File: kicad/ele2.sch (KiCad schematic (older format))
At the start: 3 parts, among them SW1 SW_Push, U1 WeMos_D1_mini, U2 HX711_module

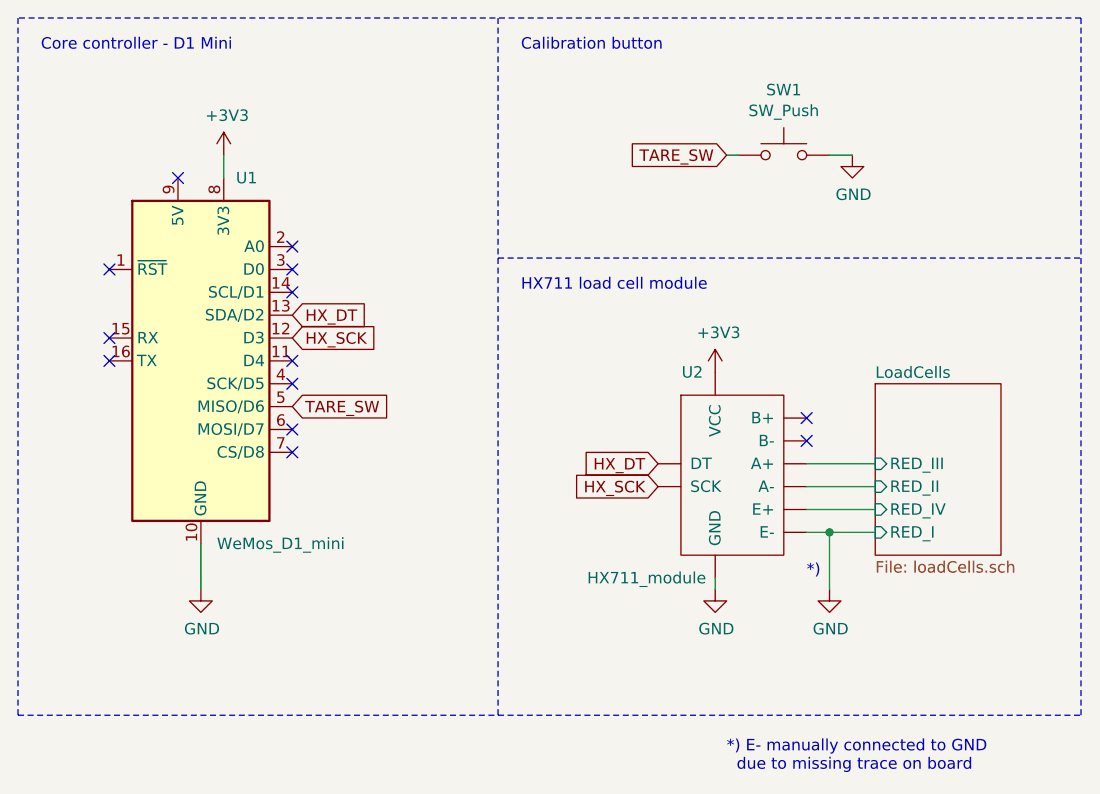
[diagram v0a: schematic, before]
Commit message: Update schematic
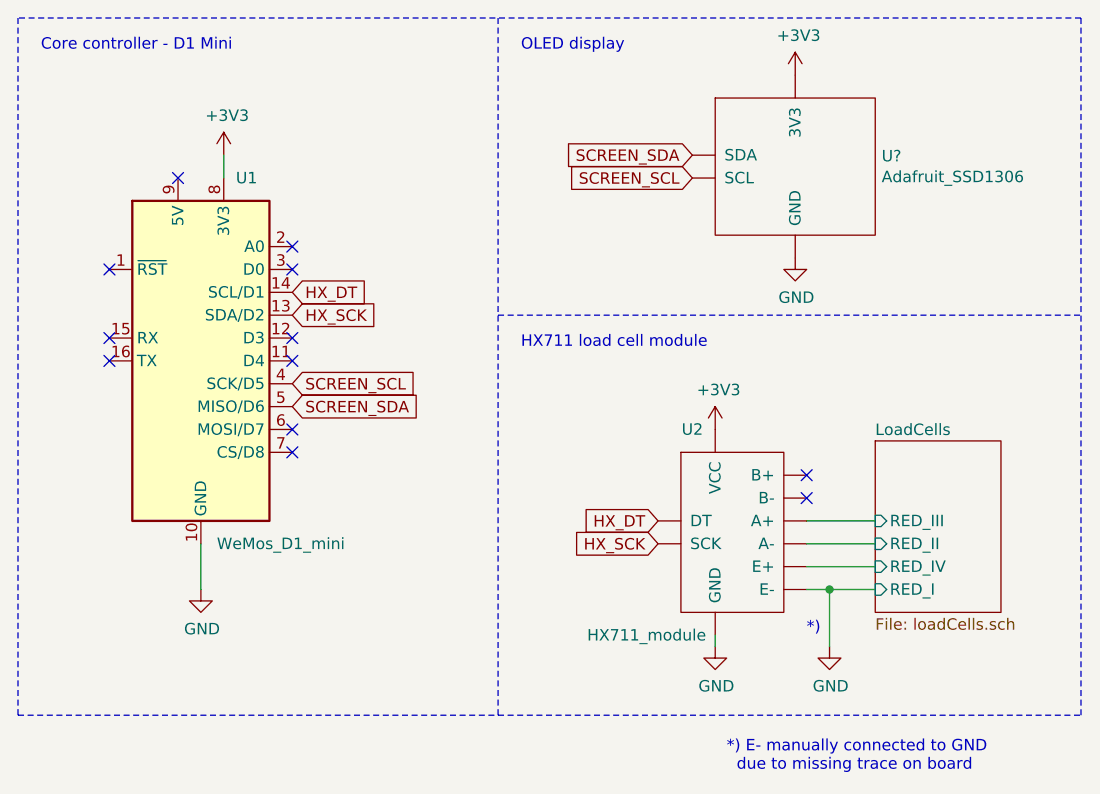
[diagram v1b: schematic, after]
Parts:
- removed SW1: SW_Push, symbol Switch:SW_Push
- added U?: Adafruit_SSD1306, symbol ele2:Adafruit_SSD1306
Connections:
- net +3V3: now also U?.~ (SDA)
- net GND: now also U?.~ (SDA)
- net HX_DT: now also U1.14 (SCL/D1); no longer U1.13 (SDA/D2)
- net HX_SCK: now also U1.13 (SDA/D2); no longer U1.12 (D3)
- net SCREEN_SCL: now reaches U1.4 (SCK/D5)
- net SCREEN_SCL: now also U?.~ (SDA)
- net TARE_SW renamed SCREEN_SDA
- net SCREEN_SDA: now also U?.~ (SDA)
- no-connect marks 13 -> 12
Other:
- note added: "OLED display"
- note removed: "Calibration button"
- moved on the sheet: U2
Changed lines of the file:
@@
 	4250 4950 4250 4750
-$Comp
-L Switch:SW_Push SW1
-U 1 1 5E80F0CB
-P 6800 3050
-F 0 "SW1" H 6800 3335 50  0000 C CNN
-F 1 "SW_Push" H 6800 3244 50  0000 C CNN
-F 2 "" H 6800 3250 50  0001 C CNN
-F 3 "~" H 6800 3250 50  0001 C CNN
-	1    6800 3050
-	1    0    0    -1
-$EndComp
-$Comp
-L power:GND #PWR?
-U 1 1 5E81082F
-P 7100 3050
-F 0 "#PWR?" H 7100 2800 50  0001 C CNN
-F 1 "GND" H 7105 2877 50  0000 C CNN
-F 2 "" H 7100 3050 50  0001 C CNN
-F 3 "" H 7100 3050 50  0001 C CNN
-	1    7100 3050
-	1    0    0    -1
-$EndComp
-Wire Wire Line
-	6550 3050 6600 3050
-Wire Wire Line
-	7000 3050 7100 3050
 $Comp
 L ele2:HX711_module U2
 U 1 1 5E815E00
-P 6550 4450
-F 0 "U2" H 6400 4900 50  0000 C CNN
-F 1 "HX711_module" H 6200 4000 50  0000 C CNN
-F 2 "" H 6550 4450 50  0001 C CNN
-F 3 "" H 6550 4450 50  0001 C CNN
-	1    6550 4450
-	1    0    0    -1
-$EndComp
-$Comp
-L power:+3V3 #PWR?
-U 1 1 5E81AC21
-P 6500 4000
-F 0 "#PWR?" H 6500 3850 50  0001 C CNN
-F 1 "+3V3" H 6515 4173 50  0000 C CNN
-F 2 "" H 6500 4000 50  0001 C CNN
-F 3 "" H 6500 4000 50  0001 C CNN
-	1    6500 4000
+P 6550 4700
+F 0 "U2" H 6400 5150 50  0000 C CNN
+F 1 "HX711_module" H 6200 4250 50  0000 C CNN
+F 2 "" H 6550 4700 50  0001 C CNN
+F 3 "" H 6550 4700 50  0001 C CNN
+	1    6550 4700
 	1    0    0    -1
 $EndComp
@@
 L power:GND #PWR?
 U 1 1 5E81C444
-P 6500 4950
-F 0 "#PWR?" H 6500 4700 50  0001 C CNN
-F 1 "GND" H 6505 4777 50  0000 C CNN
-F 2 "" H 6500 4950 50  0001 C CNN
-F 3 "" H 6500 4950 50  0001 C CNN
-	1    6500 4950
+P 6500 5200
+F 0 "#PWR?" H 6500 4950 50  0001 C CNN
+F 1 "GND" H 6505 5027 50  0000 C CNN
+F 2 "" H 6500 5200 50  0001 C CNN
+F 3 "" H 6500 5200 50  0001 C CNN
+	1    6500 5200
 	1    0    0    -1
 $EndComp
 Wire Wire Line
-	6500 4900 6500 4950
+	6500 5150 6500 5200
 NoConn ~ 4650 3450
 NoConn ~ 4650 3550
-NoConn ~ 4650 3650
-NoConn ~ 4650 4050
 NoConn ~ 4650 3950
-Text GLabel 6550 3050 0    50   Input ~ 0
-TARE_SW
-Text GLabel 4650 4150 2    50   Input ~ 0
-TARE_SW
+Text GLabel 4650 4050 2    50   Input ~ 0
+SCREEN_SCL
 NoConn ~ 4650 4250
 NoConn ~ 4650 4350
+Text GLabel 4650 3650 2    50   Input ~ 0
+HX_DT
+Text GLabel 6250 4750 0    50   Input ~ 0
+HX_SCK
 Text GLabel 4650 3750 2    50   Input ~ 0
-HX_DT
-Text GLabel 6250 4500 0    50   Input ~ 0
 HX_SCK
-Text GLabel 4650 3850 2    50   Input ~ 0
-HX_SCK
-Text GLabel 6250 4400 0    50   Input ~ 0
+Text GLabel 6250 4650 0    50   Input ~ 0
 HX_DT
 Wire Notes Line
@@
 	5550 2450 5550 5500
 Wire Notes Line
-	5550 3500 8100 3500
-Text Notes 5650 2600 0    50   ~ 0
-Calibration button
-Text Notes 5650 3650 0    50   ~ 0
+	5550 3750 8100 3750
+Text Notes 5650 3900 0    50   ~ 0
 HX711 load cell module
 Text Notes 3550 2600 0    50   ~ 0
 Core controller - D1 Mini
 Wire Wire Line
-	6900 4700 7000 4700
-Connection ~ 7000 4700
+	6900 4950 7000 4950
+Connection ~ 7000 4950
 $Comp
 L power:GND #PWR?
 U 1 1 5E83F78A
-P 7000 4950
-F 0 "#PWR?" H 7000 4700 50  0001 C CNN
-F 1 "GND" H 7005 4777 50  0000 C CNN
-F 2 "" H 7000 4950 50  0001 C CNN
-F 3 "" H 7000 4950 50  0001 C CNN
-	1    7000 4950
+P 7000 5200
+F 0 "#PWR?" H 7000 4950 50  0001 C CNN
+F 1 "GND" H 7005 5027 50  0000 C CNN
+F 2 "" H 7000 5200 50  0001 C CNN
+F 3 "" H 7000 5200 50  0001 C CNN
+	1    7000 5200
 	1    0    0    -1
 $EndComp
 Wire Wire Line
-	7000 4700 7000 4950
-Text Notes 6900 4900 0    50   ~ 0
+	7000 4950 7000 5200
+Text Notes 6900 5150 0    50   ~ 0
 *)
 Text Notes 6550 5750 0    50   ~ 0
 *) E- manually connected to GND\n  due to missing trace on board
 $Sheet
-S 7200 4050 550  750
+S 7200 4300 550  750
 U 5E83A8FB
 F0 "LoadCells" 50
 F1 "loadCells.sch" 50
-F2 "RED_II" I L 7200 4500 50
-F3 "RED_I" I L 7200 4700 50
-F4 "RED_IV" I L 7200 4600 50
-F5 "RED_III" I L 7200 4400 50
+F2 "RED_II" I L 7200 4750 50
+F3 "RED_I" I L 7200 4950 50
+F4 "RED_IV" I L 7200 4850 50
+F5 "RED_III" I L 7200 4650 50
 $EndSheet
-NoConn ~ 6900 4200
-NoConn ~ 6900 4300
+NoConn ~ 6900 4450
+NoConn ~ 6900 4550
 Wire Wire Line
-	6900 4400 7200 4400
+	6900 4650 7200 4650
 Wire Wire Line
-	6900 4500 7200 4500
+	6900 4750 7200 4750
 Wire Wire Line
-	6900 4600 7200 4600
+	6900 4850 7200 4850
 Wire Wire Line
-	7000 4700 7200 4700
+	7000 4950 7200 4950
+NoConn ~ 4650 3850
+Text GLabel 4650 4150 2    50   Input ~ 0
+SCREEN_SDA
+$Comp
+L ele2:Adafruit_SSD1306 U?
+U 1 1 5EBEA0D0
+P 6750 3100
+F 0 "U?" H 7228 3146 50  0000 L CNN
+F 1 "Adafruit_SSD1306" H 7228 3055 50  0000 L CNN
+F 2 "" H 6750 3050 50  0001 C CNN
+F 3 "" H 6750 3050 50  0001 C CNN
+	1    6750 3100
+	1    0    0    -1
+$EndComp
+$Comp
+L power:+3V3 #PWR?
+U 1 1 5E81AC21
+P 6500 4250
+F 0 "#PWR?" H 6500 4100 50  0001 C CNN
+F 1 "+3V3" H 6515 4423 50  0000 C CNN
+F 2 "" H 6500 4250 50  0001 C CNN
+F 3 "" H 6500 4250 50  0001 C CNN
+	1    6500 4250
+	1    0    0    -1
+$EndComp
+$Comp
+L power:+3V3 #PWR?
+U 1 1 5EBEDF9F
+P 6850 2700
+F 0 "#PWR?" H 6850 2550 50  0001 C CNN
+F 1 "+3V3" H 6865 2873 50  0000 C CNN
+F 2 "" H 6850 2700 50  0001 C CNN
+F 3 "" H 6850 2700 50  0001 C CNN
+	1    6850 2700
+	1    0    0    -1
+$EndComp
+$Comp
+L power:GND #PWR?
+U 1 1 5EBEE845
+P 6850 3500
+F 0 "#PWR?" H 6850 3250 50  0001 C CNN
+F 1 "GND" H 6855 3327 50  0000 C CNN
+F 2 "" H 6850 3500 50  0001 C CNN
+F 3 "" H 6850 3500 50  0001 C CNN
+	1    6850 3500
+	1    0    0    -1
+$EndComp
+Text GLabel 6400 3150 0    50   Input ~ 0
+SCREEN_SCL
+Text GLabel 6400 3050 0    50   Input ~ 0
+SCREEN_SDA
+Text Notes 5650 2600 0    50   ~ 0
+OLED display
 $EndSCHEMATC
